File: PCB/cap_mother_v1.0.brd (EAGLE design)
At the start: 55 x 55 mm, 33 parts, among them IC1 STM32L431KBU6TR, IC2 ADG701LBRJZ-REEL7, IC3 AD8605ARTZ-REEL7, IC4 AD8605ARTZ-REEL7, IC5 74HC164PW,118, U4 MIC5501-3.0YM5-TR

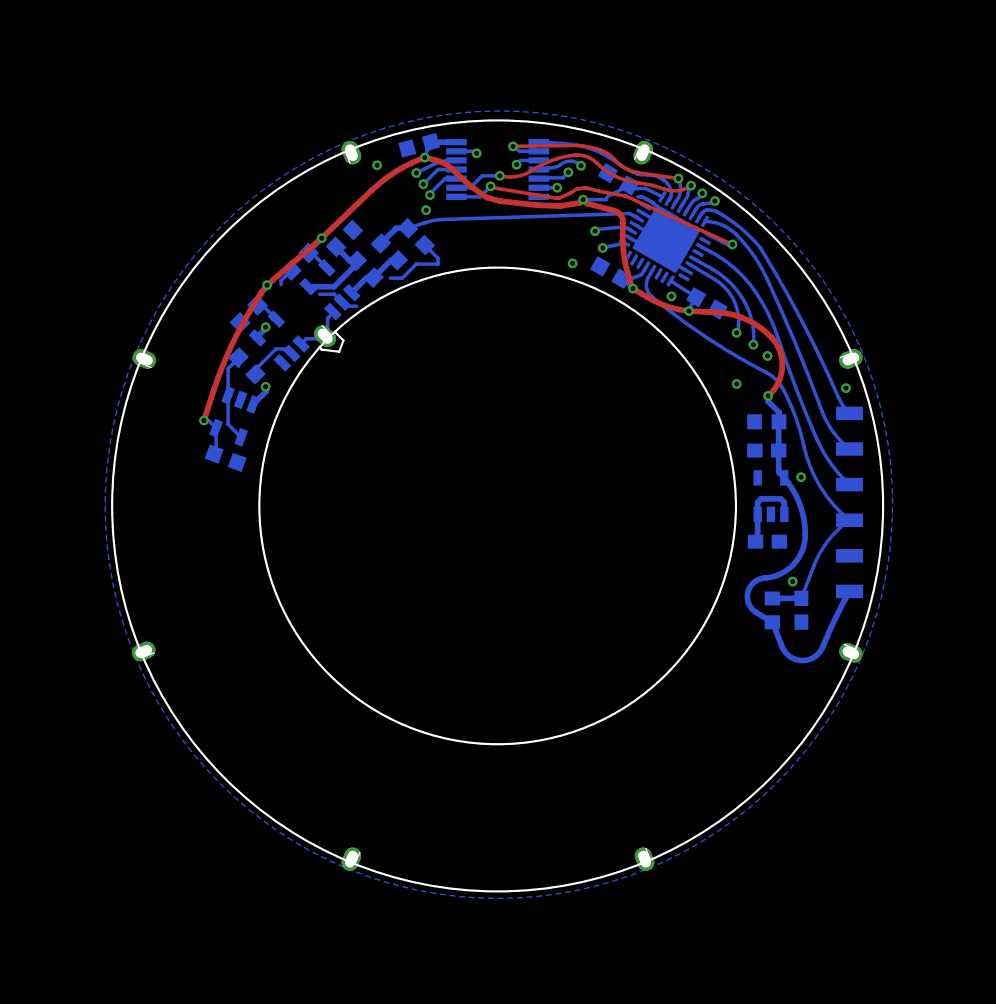
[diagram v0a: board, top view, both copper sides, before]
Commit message: final_version of v1.0 HW
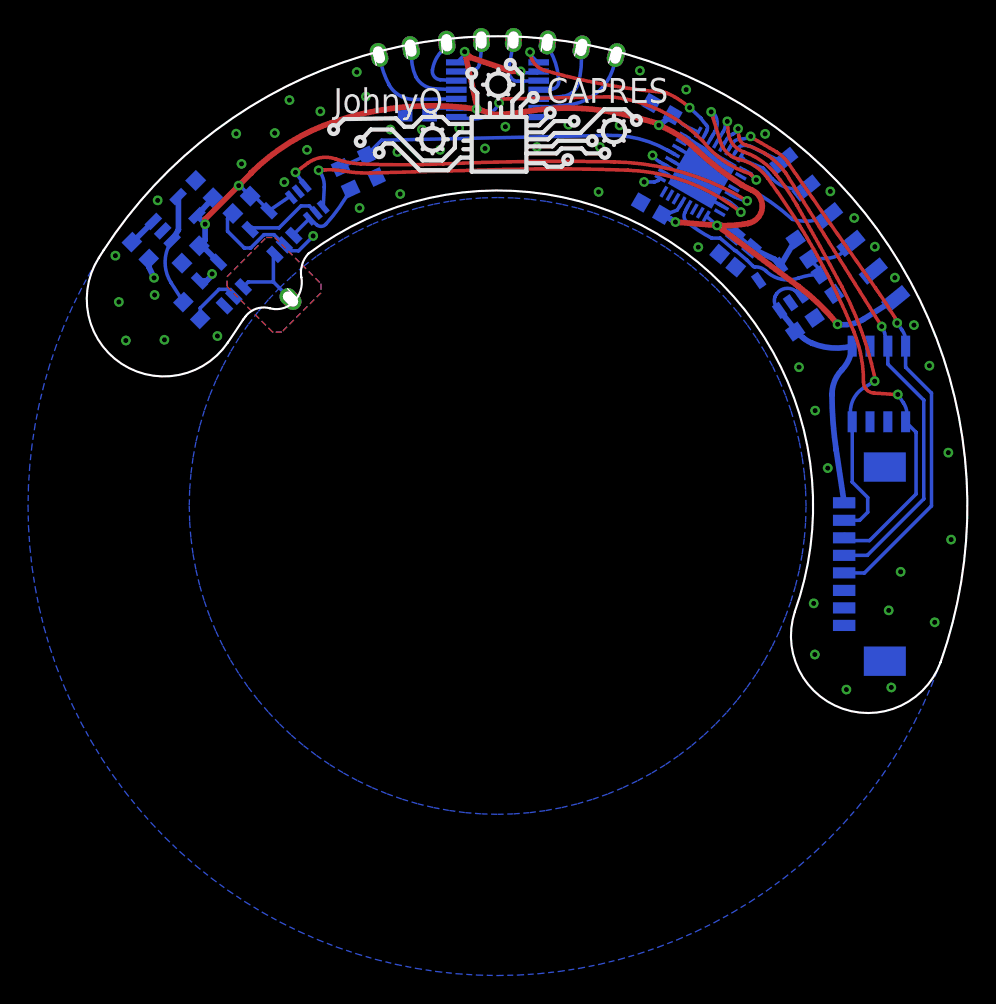
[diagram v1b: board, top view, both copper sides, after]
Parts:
- removed C11: 100n, rcl:C0603
- removed R5, R6: 100k, rcl:R0603
- added D1: SMDA05-6.TBT, SamacSys_Parts:SOIC127P600X175-8N
- added IC6: MCP40D18T-103E_LT, SamacSys_Parts:SOT65P210X110-6N
- added J1: 10114828-11108LF, SamacSys_Parts:1011482811108LF
- added R1: 0R, rcl:R0603
- moved U$5 60.0 mm to (-8.80, 33.5), turned to 14.5 degrees
- moved U$4 60.0 mm to (8.79, 33.5), turned to 345.5 degrees
- moved U$3 49.4 mm to (6.25, 34.0), turned to 349 degrees
- moved U$6 49.2 mm to (-6.45, 34.0), turned to 11 degrees
- moved U$2 32.6 mm to (3.71, 34.4), turned to 353.5 degrees
- moved U$7 32.6 mm to (-3.75, 34.4), turned to 5.3 degrees
- moved R15 25.8 mm to (21.8, 18.3), turned to 235 degrees
- moved C9 23.3 mm to (23.5, 15.8), turned to 55 degrees
- moved C5 19.3 mm to (-20.9, 22.6), turned to 225 degrees
- moved U$10 18.6 mm to (20.4, 24.6), turned to 321 degrees
- moved C20 15.7 mm to (21.9, 12.9), turned to 325 degrees
- moved U4 14.9 mm to (20.1, 15.6), turned to 55 degrees
- moved IC4 14.7 mm to (-23.0, 20.5), turned to 135 degrees
- moved U$8 12.7 mm to (-1.20, 34.6), turned to 1.8 degrees
- moved U$1 12.7 mm to (1.17, 34.6), turned to 358.2 degrees
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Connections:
- removed net T_EN: IC1.19, IC5.2
- removed net T_RST: IC1.20, IC5.9
- new net N$1: IC4.3, R1.1
- new net SCL: IC1.29, IC6.3
- new net SDA: IC1.30, IC6.4
- net +3V3: now also IC5.2, IC5.9, IC6.1; no longer C11.2
- net BIAS_IN: now also R1.2; no longer IC4.3
- net CAN1_RX: now also D1.3, J1.4
- net CAN1_TX: now also D1.4, J1.5
- net GND: now also D1.6, D1.7, IC6.2, J1.8, J1.MP1, J1.MP2; no longer C11.1, R6.2
- net IN-: now also IC6.5; no longer R5.1, R6.1
- net OUT_: now also IC6.6; no longer R5.2
- net USART1_RX: now also D1.8, IC1.20, J1.2; no longer IC1.30
- net USART1_TX: now also D1.5, IC1.19, J1.3; no longer IC1.29
- net VDD: now also D1.1, J1.1
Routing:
- net S04: track 63.3 -> 7.07 mm, vias 1 -> 0
- net S03: track 60.7 -> 6.83 mm, vias 1 -> 0
- net S05: track 46.1 -> 4.96 mm, vias 1 -> 0
- net S02: track 46.2 -> 5.85 mm, vias 1 -> 0
- net CAN1_TX: track 1.96 -> 41.3 mm, vias 1 -> 2
- net CAN1_RX: track 1.69 -> 40.3 mm, vias 1 -> 2
- net SCL: track 0.00 -> 35.4 mm, vias 0 -> 2
- net SDA: track 0.00 -> 34.7 mm, vias 0 -> 2
- net USART1_TX: track 7.86 -> 42.0 mm, vias 1 -> 2
- net USART1_RX: track 6.26 -> 35.9 mm, vias 1 -> 2
- net S01: track 27.7 -> 4.33 mm, vias 1 -> 0
- net S06: track 27.3 -> 4.02 mm, vias 1 -> 0
- net T_RST: track 19.5 -> 0.00 mm, vias 2 -> 0
- net T_EN: track 16.2 -> 0.00 mm, vias 2 -> 0
- net RST: track 32.7 -> 16.7 mm
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- added copper zone on layer 1, net GND
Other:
- board size 55 x 55 mm -> 62.8 x 48.3 mm
- board text added: "3V3"
- board text added: "CLK"
- board text added: "GND"
- board text added: "IO"
- board text added: "RST"
- board text added: "SWO"
